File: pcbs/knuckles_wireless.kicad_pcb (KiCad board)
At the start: 2 copper layers, 130.3 x 107.9 mm, 121 parts

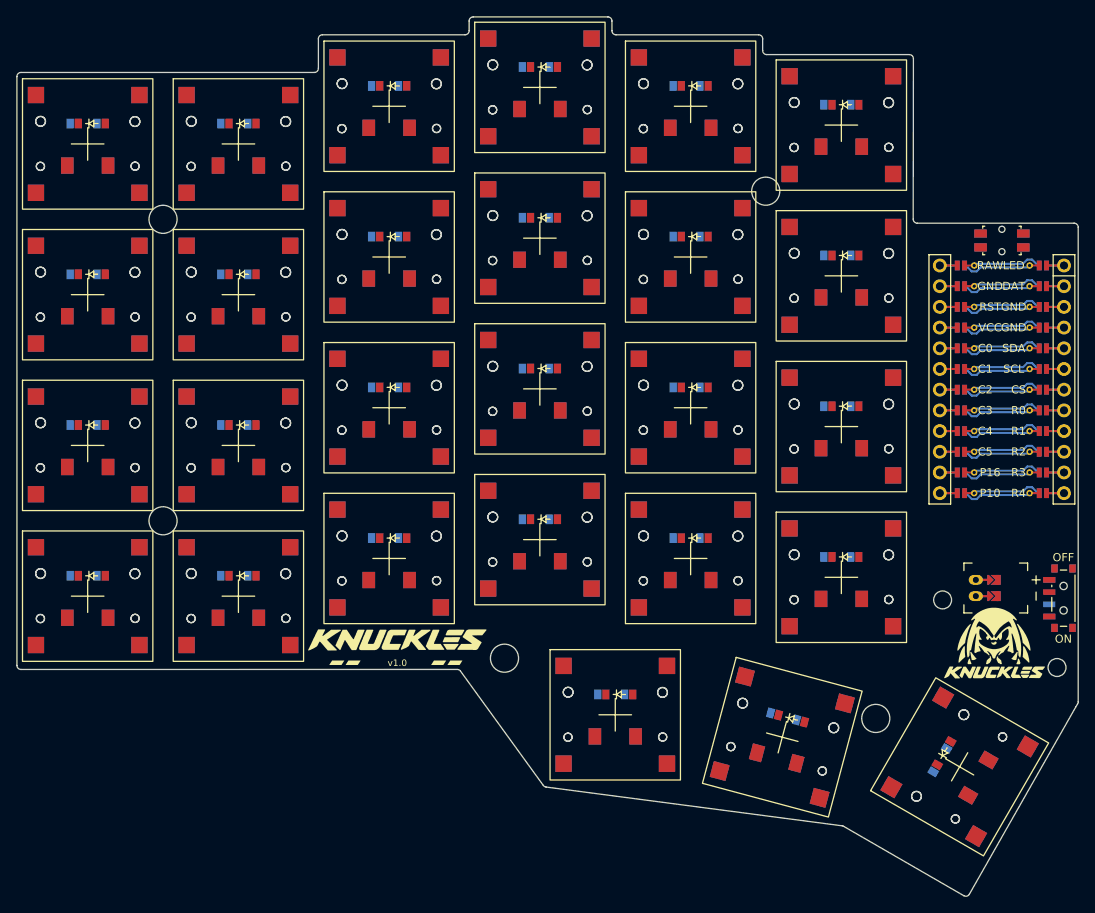
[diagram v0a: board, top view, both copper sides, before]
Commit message: Archive ordered wireless PCB and manufacturing files
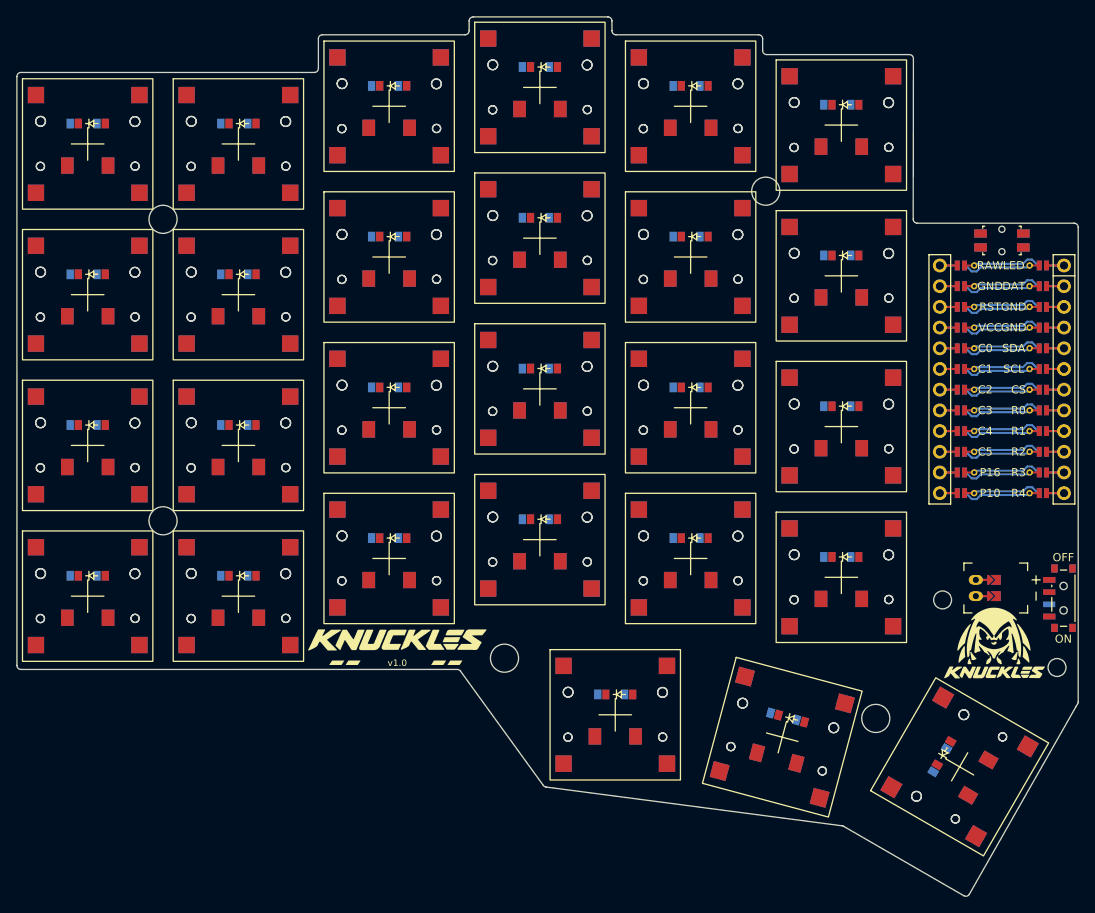
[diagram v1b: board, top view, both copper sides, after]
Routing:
- net (no net): track 333.1 -> 0.00 mm
- net GND: track 0.00 -> 28.9 mm
- net C3: track 0.00 -> 9.64 mm
- net C1: track 0.00 -> 9.64 mm
- net VCC: track 0.00 -> 9.64 mm
- net RST: track 0.00 -> 9.64 mm
- net RAW: track 0.00 -> 9.64 mm
- net P16: track 0.00 -> 9.64 mm
- net P10: track 0.00 -> 9.64 mm
- net C5: track 0.00 -> 9.64 mm
- net C4: track 0.00 -> 9.64 mm
- net C2: track 0.00 -> 9.64 mm
- net C0: track 0.00 -> 9.64 mm
- net SDA: track 0.00 -> 9.63 mm
- net R3: track 0.00 -> 9.63 mm
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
